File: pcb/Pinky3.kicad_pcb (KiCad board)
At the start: 2 copper layers, 137 x 100.9 mm, 65 parts, among them J1 MJ-4PP-9, P1 i2c-pin, P2 i2c-pin, SW1 RESET_SW, SW10 SW_PUSH, SW11 SW_PUSH, SW12 SW_PUSH, SW13 SW_PUSH, SW14 SW_PUSH, SW15 SW_PUSH, SW16 SW_PUSH, SW17 SW_PUSH, SW18 SW_PUSH, SW19 SW_PUSH, SW2 SW_PUSH, SW20 SW_PUSH, SW21 SW_PUSH, SW22 SW_PUSH, SW23 SW_PUSH, SW24 SW_PUSH, SW25 SW_PUSH, SW26 SW_PUSH, SW3 SW_PUSH, SW4 SW_PUSH, SW5 SW_PUSH, SW6 SW_PUSH, SW7 SW_PUSH, SW8 SW_PUSH, SW9 SW_PUSH, U1 ProMicro

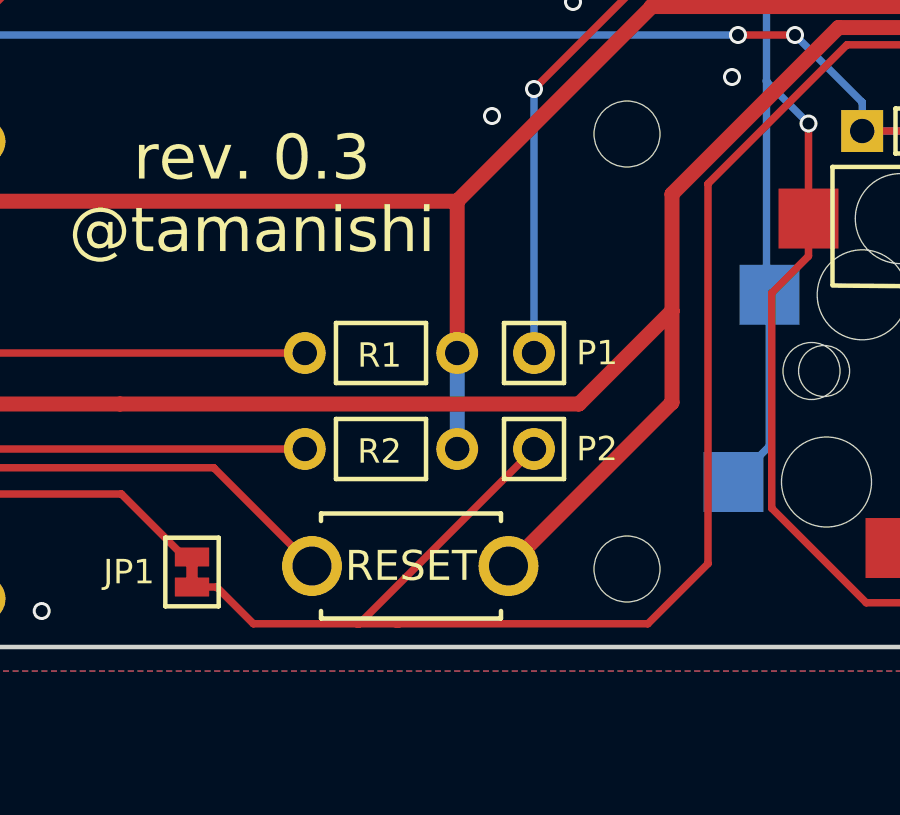
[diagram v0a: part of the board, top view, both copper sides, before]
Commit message: tweak
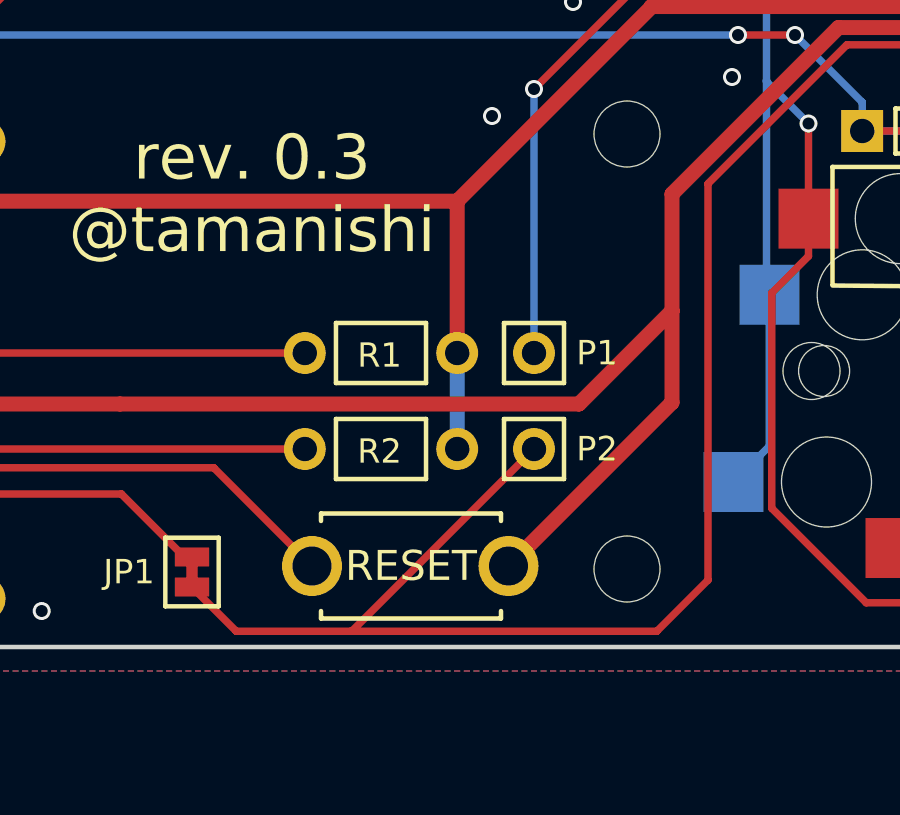
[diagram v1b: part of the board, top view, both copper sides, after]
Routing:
- net Net-(J1-PadB): track 125.4 -> 126.1 mm
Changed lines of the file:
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@@
     (thickness 1.6)
     (drawings 163)
-    (tracks 955)
+    (tracks 953)
     (zones 0)
     (modules 65)
@@
     (38 B.Mask user)
     (39 F.Mask user)
-    (40 Dwgs.User user hide)
+    (40 Dwgs.User user)
     (41 Cmts.User user)
     (42 Eco1.User user)
@@
   (segment (start 164.9 107.95) (end 164.9 105.5) (width 0.25) (layer F.Cu) (net 28))
   (segment (start 102.831509 116.226489) (end 98.2 120.857998) (width 0.25) (layer F.Cu) (net 29))
-  (segment (start 98.2 133.521002) (end 96.196001 135.525001) (width 0.25) (layer F.Cu) (net 29))
-  (segment (start 98.2 120.857998) (end 98.2 133.521002) (width 0.25) (layer F.Cu) (net 29))
-  (segment (start 81.8215 134.30038) (end 81 134.30038) (width 0.25) (layer F.Cu) (net 29) (status 20))
-  (segment (start 83.046121 135.525001) (end 81.8215 134.30038) (width 0.25) (layer F.Cu) (net 29))
-  (segment (start 87.9 135.525001) (end 87.774999 135.525001) (width 0.25) (layer F.Cu) (net 29))
-  (segment (start 96.196001 135.525001) (end 87.9 135.525001) (width 0.25) (layer F.Cu) (net 29))
-  (segment (start 86.574999 135.525001) (end 86.5 135.525001) (width 0.25) (layer F.Cu) (net 29))
-  (segment (start 92.4 129.7) (end 86.574999 135.525001) (width 0.25) (layer F.Cu) (net 29) (status 10))
-  (segment (start 86.5 135.525001) (end 83.046121 135.525001) (width 0.25) (layer F.Cu) (net 29))
-  (segment (start 87.9 135.525001) (end 86.5 135.525001) (width 0.25) (layer F.Cu) (net 29))
   (segment (start 166.503122 116.196878) (end 173 109.7) (width 0.25) (layer F.Cu) (net 29))
   (segment (start 173 109.7) (end 173.4 109.7) (width 0.25) (layer F.Cu) (net 29))
@@
   (segment (start 102.831509 116.226489) (end 162.773511 116.226489) (width 0.25) (layer F.Cu) (net 29))
   (segment (start 173.4 109.7) (end 173.4 103.75) (width 0.25) (layer F.Cu) (net 29))
+  (segment (start 81.015121 134.315501) (end 81 134.315501) (width 0.25) (layer F.Cu) (net 29))
+  (segment (start 98.2 134.071002) (end 96.496001 135.775001) (width 0.25) (layer F.Cu) (net 29))
+  (segment (start 82.474621 135.775001) (end 81.015121 134.315501) (width 0.25) (layer F.Cu) (net 29))
+  (segment (start 98.2 120.857998) (end 98.2 134.071002) (width 0.25) (layer F.Cu) (net 29))
+  (segment (start 92.4 129.7) (end 86.324999 135.775001) (width 0.25) (layer F.Cu) (net 29))
+  (segment (start 86.324999 135.775001) (end 86.3 135.775001) (width 0.25) (layer F.Cu) (net 29))
+  (segment (start 86.3 135.775001) (end 82.474621 135.775001) (width 0.25) (layer F.Cu) (net 29))
+  (segment (start 96.496001 135.775001) (end 86.3 135.775001) (width 0.25) (layer F.Cu) (net 29))
   (via (at 157.9 81.9) (size 0.6) (drill 0.4) (layers F.Cu B.Cu) (net 30))
   (segment (start 52.432 118.1436) (end 49.892 118.1436) (width 0.5) (layer B.Cu) (net 30) (status 30))
